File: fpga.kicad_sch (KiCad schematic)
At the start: 29 parts, among them U10 P0082_BOTTOMMOUNT, U11 SN75160BDW, U12 SN75160BDW, U13 SN75160BDW, U14 SN75160BDW

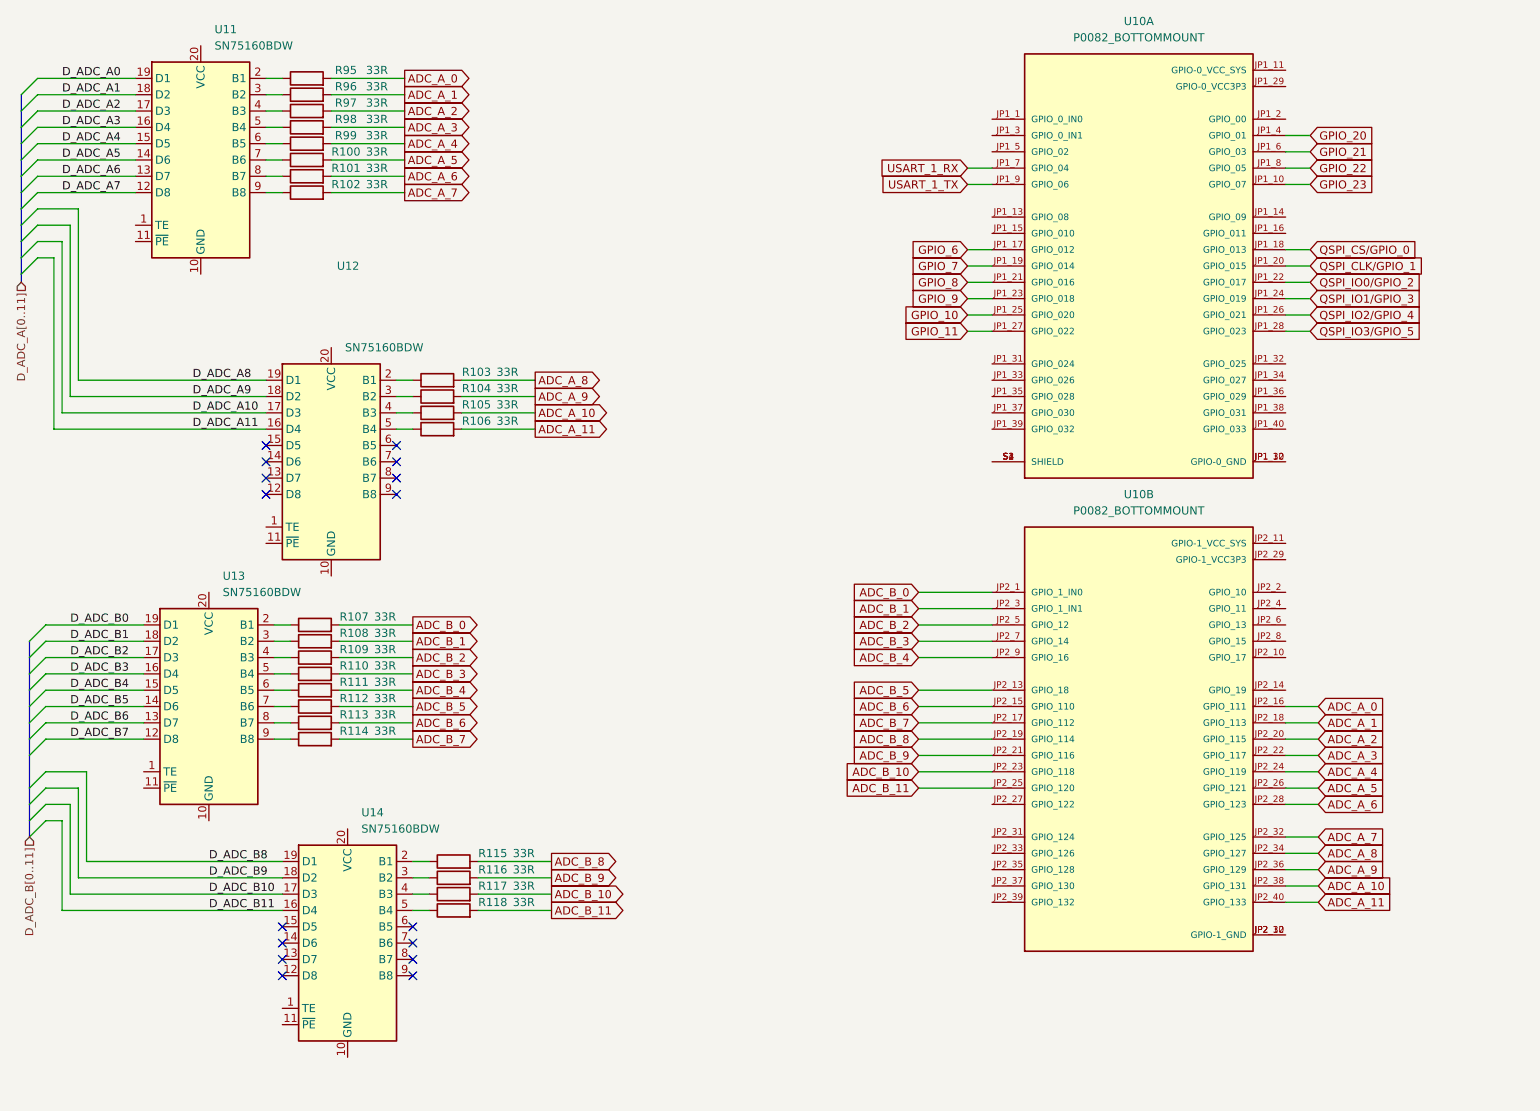
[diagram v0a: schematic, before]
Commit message: Save work on simplifying the desing
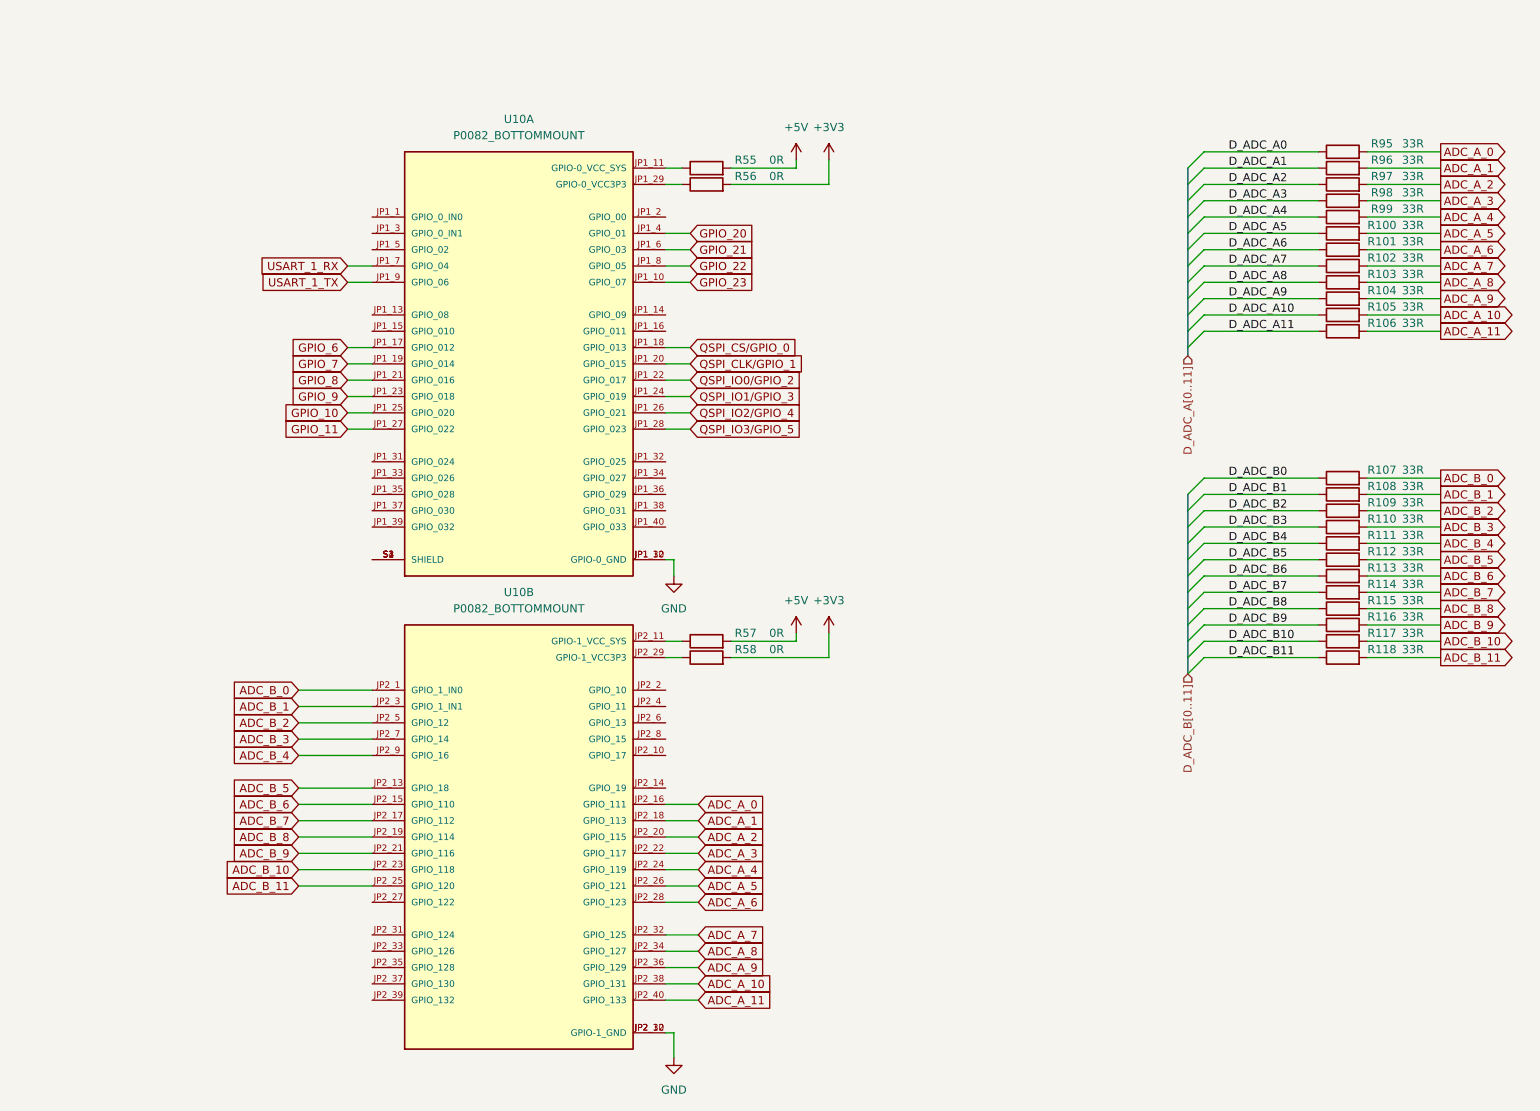
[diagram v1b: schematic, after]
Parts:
- removed U11, U12, U13, U14: SN75160BDW, Package_SO:SOIC-20W_7.5x12.8mm_P1.27mm, symbol Interface:SN75160BDW
- added R55, R56, R57, R58: 0R, Resistor_SMD:R_0402_1005Metric_Pad0.72x0.64mm_HandSolder, symbol Device:R
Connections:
- net D_ADC_A0: now also R95.1
- net D_ADC_A1: now also R96.1
- net D_ADC_A10: now also R105.1
- net D_ADC_A11: now also R106.1
- net D_ADC_A2: now also R97.1
- net D_ADC_A3: now also R98.1
- net D_ADC_A4: now also R99.1
- net D_ADC_A5: now also R100.1
- net D_ADC_A6: now also R101.1
- net D_ADC_A7: now also R102.1
- net D_ADC_A8: now also R103.1
- net D_ADC_A9: now also R104.1
- net D_ADC_B0: now also R107.1
- net D_ADC_B1: now also R108.1
- net D_ADC_B10: now also R117.1
- net D_ADC_B11: now also R118.1
- net D_ADC_B2: now also R109.1
- net D_ADC_B3: now also R110.1
- net D_ADC_B4: now also R111.1
- net D_ADC_B5: now also R112.1
- net D_ADC_B6: now also R113.1
- net D_ADC_B7: now also R114.1
- net D_ADC_B8: now also R115.1
- net D_ADC_B9: now also R116.1
- net at U10.JP1_11 (GPIO-0_VCC_SYS): now also R55.1
- net GND: now reaches U10.JP1_12 (GPIO-0_GND), U10.JP1_30 (GPIO-0_GND)
- net GND: now also U10.JP2_12 (GPIO-1_GND), U10.JP2_30 (GPIO-1_GND)
- net at U10.JP1_29 (GPIO-0_VCC3P3): now also R56.1
- net at U10.JP2_11 (GPIO-1_VCC_SYS): now also R57.1
- net at U10.JP2_29 (GPIO-1_VCC3P3): now also R58.1
- new net +3V3: R56.2, R58.2
- new net +5V: R55.2, R57.2
- no-connect marks 16 -> 0
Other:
- moved on the sheet: R100, R101, R102, R103, R104, R105, R106, R107, R108, R109, R110, R111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
